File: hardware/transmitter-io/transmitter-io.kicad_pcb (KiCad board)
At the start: 2 copper layers, 60 x 60 mm, 22 parts, among them J1 IO EXTENSION, J2 DIMMER_B, J5 12V_A, J6 12V_B, U1 LM317T, U2 74LS164, U3 TLC7226A, U4 LM324A

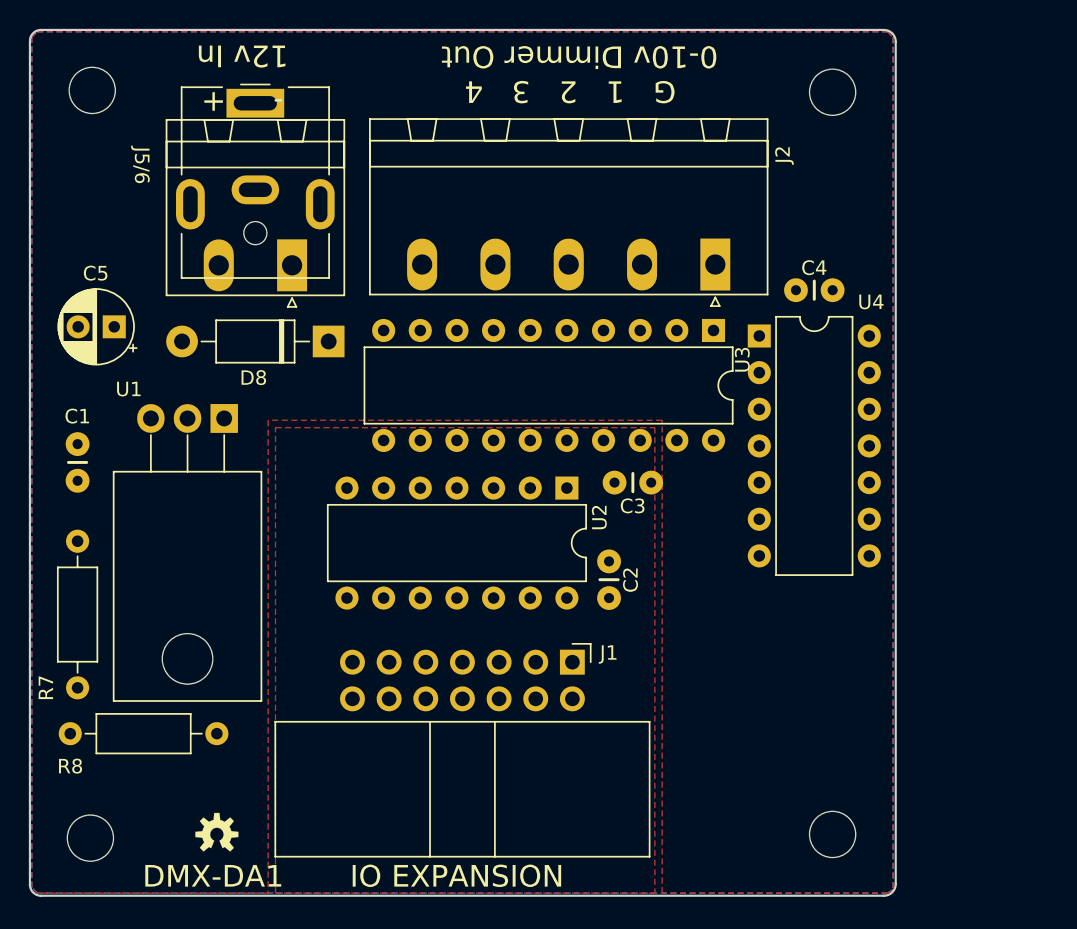
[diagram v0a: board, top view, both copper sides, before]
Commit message: Add analog, pwm, dmx, and io boards. Still needs work.
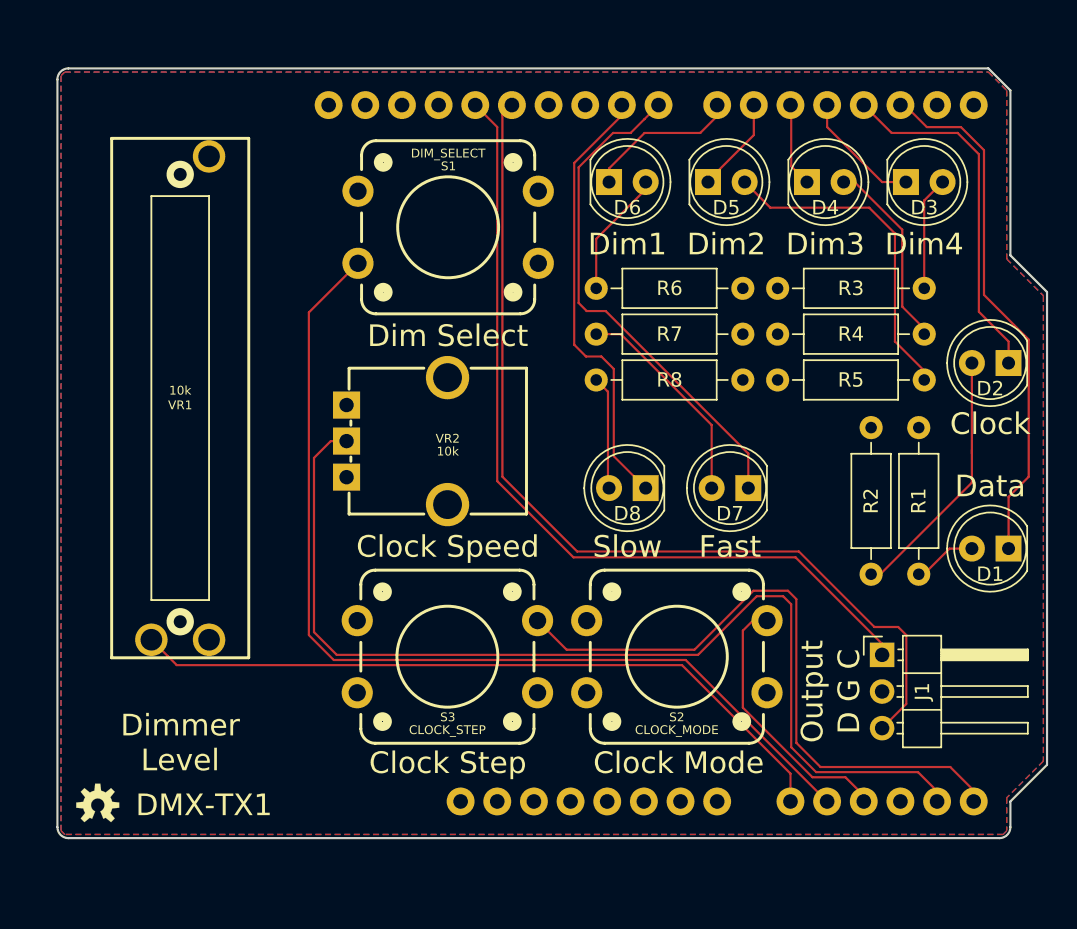
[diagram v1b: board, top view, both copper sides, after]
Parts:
- removed C1, C2, C3, C4: .01uF, Capacitors:CAP-PTH-2.54
- removed C5: 10uF, Capacitor_THT:CP_Radial_D5.0mm_P2.50mm
- removed J2: DIMMER_B, Connector_Phoenix_MSTB:PhoenixContact_MSTBA_2,5_5-G-5,08_1x05_P5.08mm_Horizontal
- removed J5: 12V_A, Connector_BarrelJack:BarrelJack_CUI_PJ-063AH_Horizontal
- removed J6: 12V_B, Connector_Phoenix_MSTB:PhoenixContact_MSTBA_2,5_2-G-5,08_1x02_P5.08mm_Horizontal
- removed MH1, MH2, MH3, MH4: MountingHole, MountingHole:MountingHole_3.2mm_M3
- removed U1: LM317T, Package_TO_SOT_THT:TO-220-3_Horizontal_TabDown
- removed U2: 74LS164, Package_DIP:DIP-14_W7.62mm
- removed U3: TLC7226A, Package_DIP:DIP-20_W7.62mm
- removed U4: LM324A, Package_DIP:DIP-14_W7.62mm
- added A1: Arduino_UNO_R3, footprints:ARDUINO_R3_NO_HOLES, F.Cu at (150.6, 89.9)
- added D1: DATA, LED_THT:LED_D5.0mm, F.Cu at (182.2, 96.5)
- added D2: CLOCK, LED_THT:LED_D5.0mm, F.Cu at (182.2, 83.7)
- added D3: DIM3, LED_THT:LED_D5.0mm, F.Cu at (175.1, 71.1)
- added D4: DIM2, LED_THT:LED_D5.0mm, F.Cu at (168.3, 71.1)
- added D5: DIM1, LED_THT:LED_D5.0mm, F.Cu at (161.4, 71.1)
- added D6: DIM0, LED_THT:LED_D5.0mm, F.Cu at (154.6, 71.1)
- added D7: CLK_FST, LED_THT:LED_D5.0mm, F.Cu at (164.2, 92.3)
- added R1: 330, Resistor_THT:R_Axial_DIN0207_L6.3mm_D2.5mm_P10.16mm_Horizontal, F.Cu at (176.0, 88.1)
- added R2: 330, Resistor_THT:R_Axial_DIN0207_L6.3mm_D2.5mm_P10.16mm_Horizontal, F.Cu at (172.7, 88.1)
- added R3: 330, Resistor_THT:R_Axial_DIN0207_L6.3mm_D2.5mm_P10.16mm_Horizontal, F.Cu at (166.2, 78.5)
- added R4: 330, Resistor_THT:R_Axial_DIN0207_L6.3mm_D2.5mm_P10.16mm_Horizontal, F.Cu at (166.2, 81.7)
- added R5: 330, Resistor_THT:R_Axial_DIN0207_L6.3mm_D2.5mm_P10.16mm_Horizontal, F.Cu at (166.2, 84.8)
- added R6: 330, Resistor_THT:R_Axial_DIN0207_L6.3mm_D2.5mm_P10.16mm_Horizontal, F.Cu at (163.8, 78.5)
- added S1: DIM_SELECT, Switches:TACTILE_SWITCH_PTH_12MM, F.Cu at (143.4, 74.3)
- added S2: CLOCK_MODE, Switches:TACTILE_SWITCH_PTH_12MM, F.Cu at (159.3, 104.0)
- added S3: CLOCK_STEP, Switches:TACTILE_SWITCH_PTH_12MM, F.Cu at (143.4, 104.0)
- added VR1: 10k, Resistors:SLIDER-SMALL, F.Cu at (124.8, 86.1)
- added VR2: 10k, Resistors:POT-PTH-ALPS, F.Cu at (143.4, 89.1)
- D8: value 1N5819 -> CLK_SLO; footprint Diode_THT:D_DO-41_SOD81_P10.16mm_Horizontal -> LED_THT:LED_D5.0mm
- J1: value IO EXTENSION -> Output; footprint Connector_IDC:IDC-Header_2x07_P2.54mm_Horizontal -> Connector_PinHeader_2.54mm:PinHeader_1x03_P2.54mm_Horizontal
- R7: value 390 -> 330
- R8: value 2.7k -> 330
- moved R7 52.2 mm to (163.8, 81.7), turned to 180 degrees
- moved R8 43.9 mm to (163.8, 84.8)
- moved D8 24.2 mm to (157.1, 92.3)
- moved J1 21.5 mm to (173.5, 103.9), turned to 0 degrees
- moved G*** 15.5 mm to (120.1, 109.5)
- moved ? 8.50 mm to (119.1, 114.3)
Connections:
- D8 pad 1: Net-(D8-Pad1) -> /~CLK_SLO
- J1 pad 1: +5V -> /RXCLK
- J1 pad 2: +5V -> GND
- J1 pad 3: /~WR -> /RX
- R7 pad 1: Net-(R7-Pad1) -> +5V
- R7 pad 2: +10V -> Net-(D7-Pad2)
- R8 pad 1: GND -> +5V
- R8 pad 2: Net-(R7-Pad1) -> Net-(D8-Pad2)
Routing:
- net /A4: track 0.00 -> 72.4 mm
- net /A1: track 0.00 -> 68.7 mm
- net /RX: track 0.00 -> 65.7 mm
- net /RXCLK: track 0.00 -> 59.4 mm
- net /A0: track 0.00 -> 50.1 mm
- net /A5: track 0.00 -> 46.0 mm
- net /~DATA: track 0.00 -> 36.6 mm
- net /~CLK_FST: track 0.00 -> 35.2 mm
- net /~CLK_SLO: track 0.00 -> 30.6 mm
- net /~CLOCK: track 0.00 -> 24.7 mm
- net Net-(D5-Pad2): track 0.00 -> 22.9 mm
- net /A2: track 0.00 -> 18.6 mm
- net Net-(D2-Pad2): track 0.00 -> 18.2 mm
- net Net-(D7-Pad2): track 0.00 -> 15.0 mm
- net Net-(D4-Pad2): track 0.00 -> 13.3 mm
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- removed copper zone on F.Cu, net +10V
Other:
- board size 60 x 60 mm -> 68.6 x 53.3 mm
- net class Power added: clearance 0.1524, trace_width 0.3048, via_dia 1.27, via_drill 0.635
- board text added: "Clock"
- board text added: "Clock Mode"
- board text added: "Clock Speed"
- board text added: "Clock Step"
- board text added: "D G C"
- board text added: "DMX-TX1"
- board text added: "DMX-TX1, Rev 1.2 Crazy Giraffe Software"
- board text added: "Data"
- board text added: "Dim Select"
- board text added: "Dim1"
- board text added: "Dim2"
- board text added: "Dim3"
- board text added: "Dim4"
- board text added: "Dimmer Level"
- board text added: "Fast"
- board text added: "Output"
- board text added: "Slow"
- board text removed: "- +"
- board text removed: "12v In"
- board text removed: "DMX-DA1"
- board text removed: "DMX-DA1, Rev 1.1 Crazy Giraffe Software"
- board text removed: "G 1 2 3 4 0-10v Dimmer Out"
- board text removed: "IO EXPANSION"
- board text removed: "J5/6"
